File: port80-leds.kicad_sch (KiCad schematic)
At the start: 19 parts, among them U6001 SN74AC7541_VQFN, U6009 SN74AC7541_VQFN

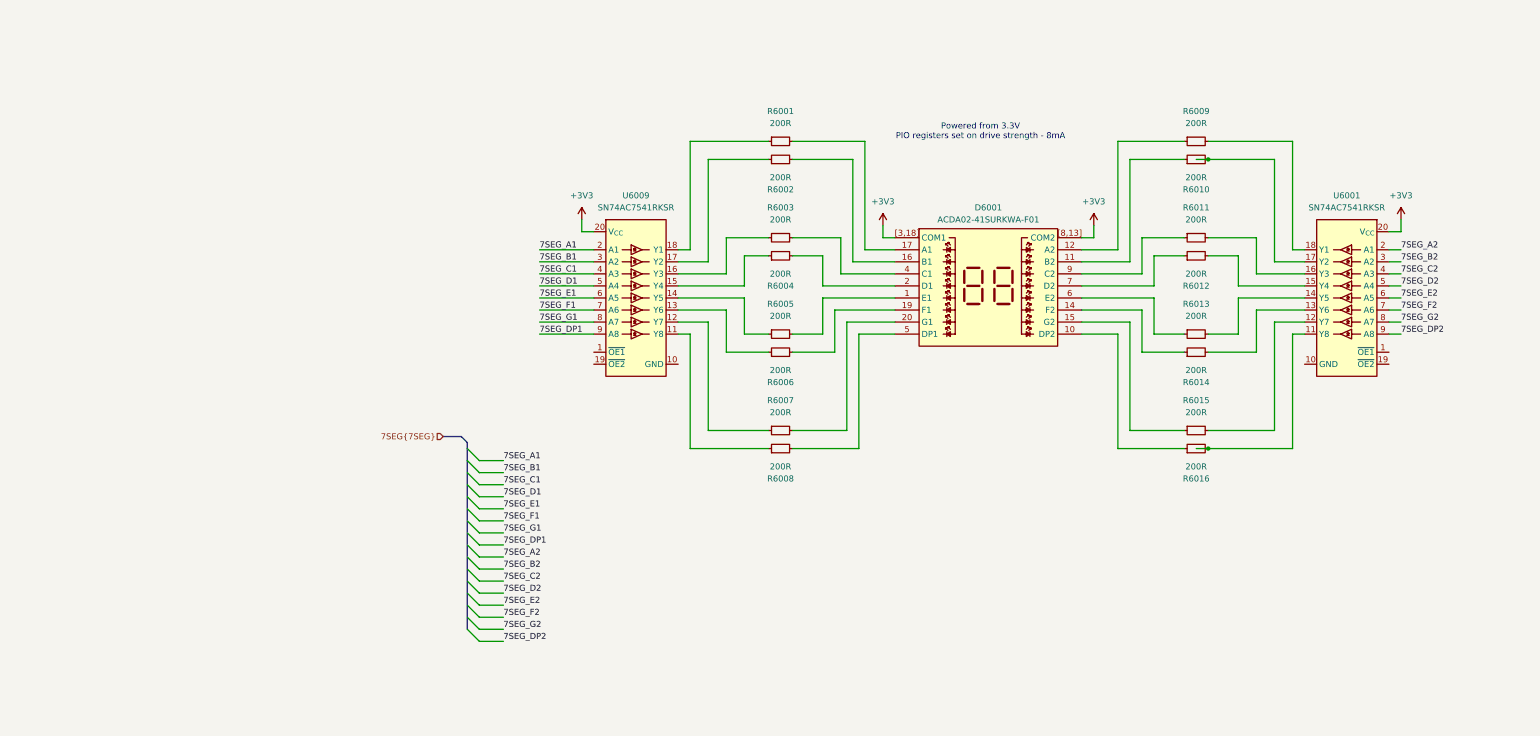
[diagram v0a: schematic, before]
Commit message: [#103224] Route 7segment buffers, fix minor typos,add TODO list
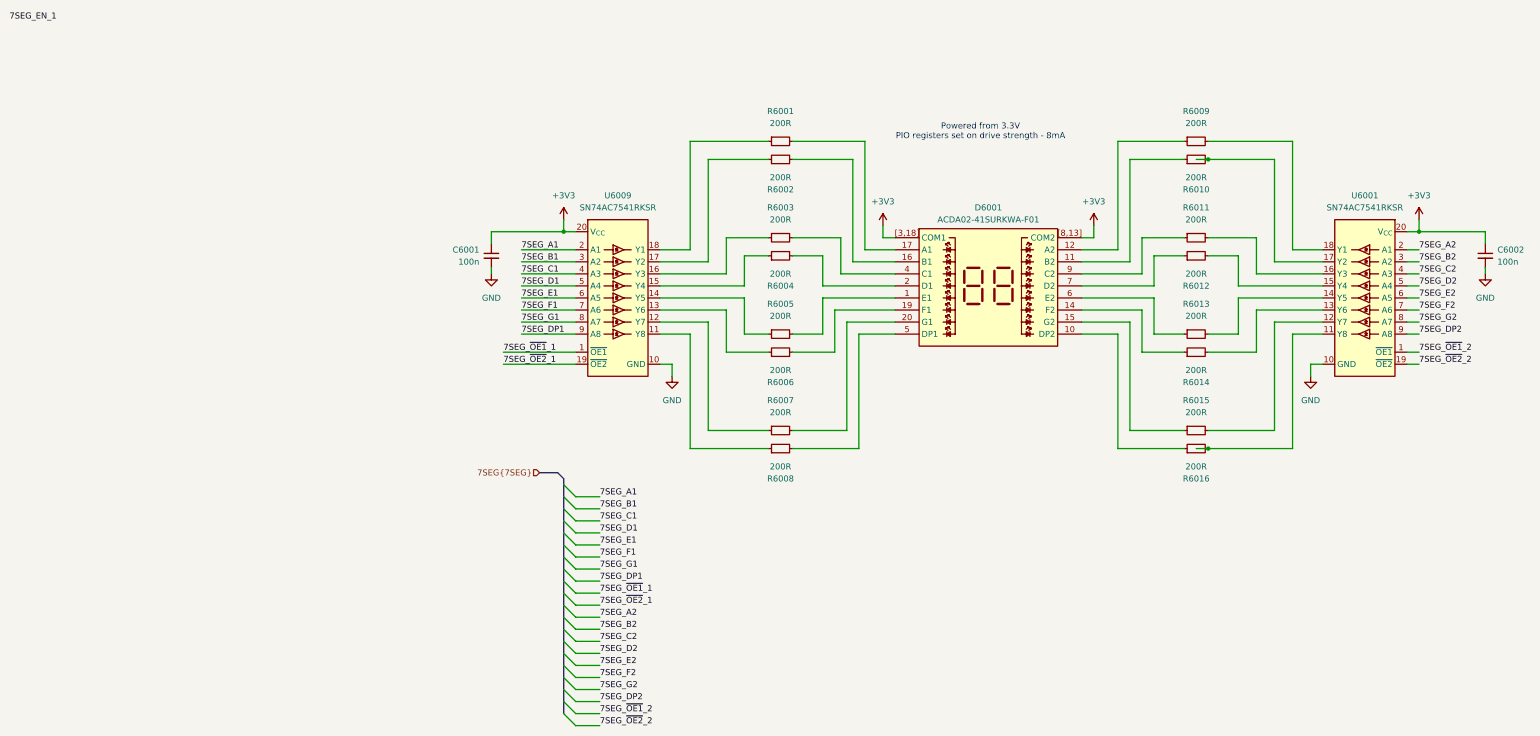
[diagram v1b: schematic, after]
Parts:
- added C6001, C6002: C_100n_0402, antmicro-footprints:C_0402_1005Metric, symbol Capacitors0402:C_100n_0402
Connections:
- net +3V3: now also C6001.1, C6002.1
- net 7SEG_~{OE1}_2: now reaches U6001.1 (~{OE1})
- net GND: now reaches U6001.10 (GND), U6001.21 (GND)
- net GND: now also U6009.10 (GND), U6009.21 (GND), C6001.2, C6002.2
- net 7SEG_~{OE2}_2: now reaches U6001.19 (~{OE2})
- net 7SEG_~{OE1}_1: now reaches U6009.1 (~{OE1})
- net 7SEG_~{OE2}_1: now reaches U6009.19 (~{OE2})
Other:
- moved on the sheet: U6001, U6009
